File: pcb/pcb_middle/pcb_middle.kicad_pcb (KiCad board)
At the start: 2 copper layers, 37 x 37 mm, 25 parts, among them J1 MicroLab, J2 Pump 1, J3 Pump 2, Q1 NX7002BKR, Q2 NX7002BKR, Q3 NX7002BKR

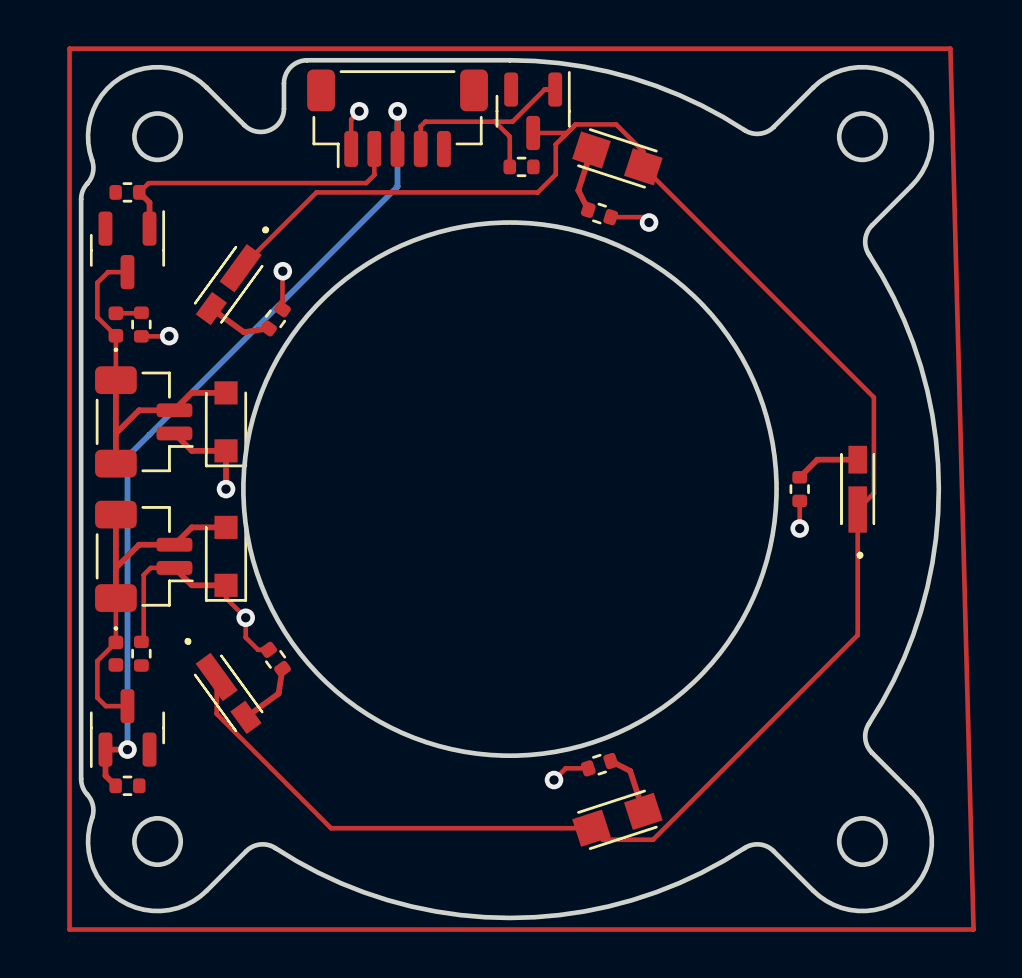
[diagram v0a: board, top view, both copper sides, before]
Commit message: fin
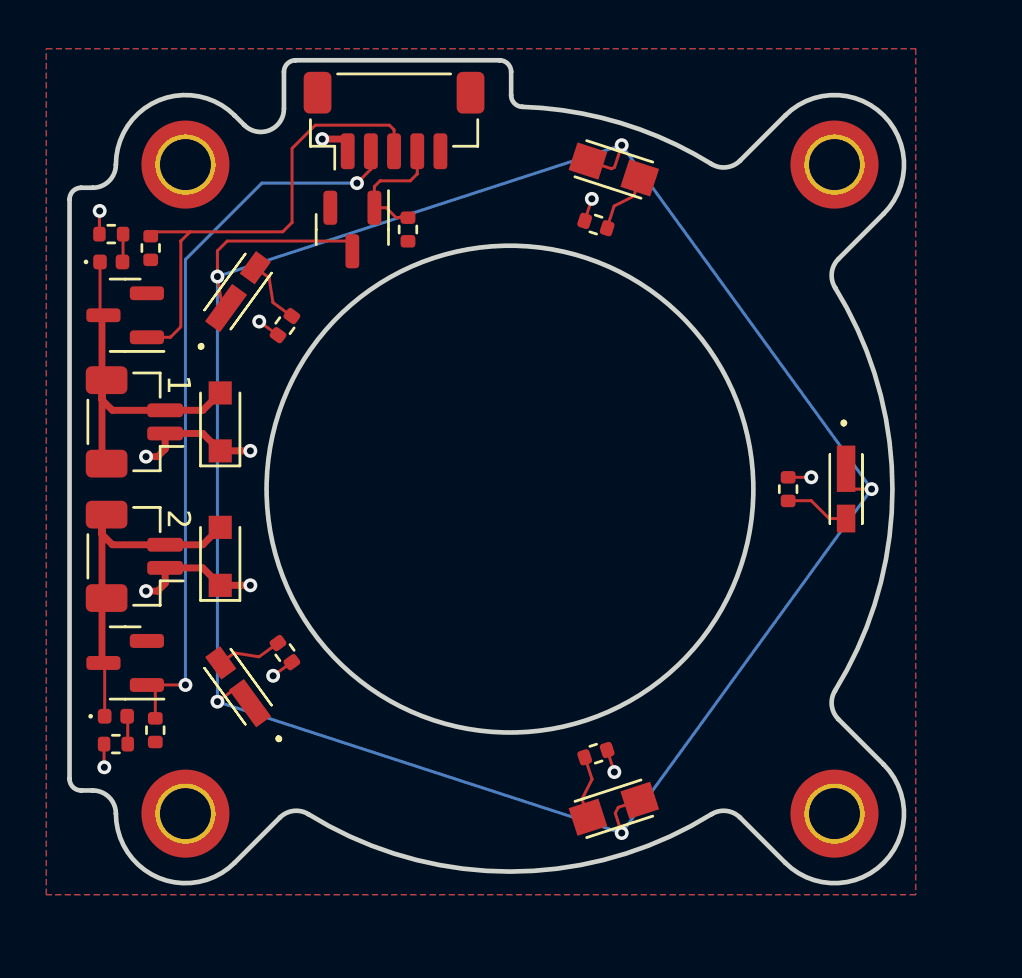
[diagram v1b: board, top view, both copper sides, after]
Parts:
- added H1: M2, MountingHole:MountingHole_2.2mm_M2_DIN965_Pad_TopOnly, F.Cu at (14.0, -14.0)
- added H2: M2, MountingHole:MountingHole_2.2mm_M2_DIN965_Pad_TopOnly, F.Cu at (14.0, 14.0)
- added H3: M2, MountingHole:MountingHole_2.2mm_M2_DIN965_Pad_TopOnly, F.Cu at (-14.0, 14.0)
- added H4: M2, MountingHole:MountingHole_2.2mm_M2_DIN965_Pad_TopOnly, F.Cu at (-14.0, -14.0)
- moved R7 23.2 mm to (-15.3, 10.4), turned to -90 degrees
- moved R2 23.2 mm to (-15.5, -10.4), turned to -90 degrees
- moved R9 18.1 mm to (-17.2, -11.0), turned to 0 degrees
- moved R10 18.1 mm to (-17.0, 11.0), turned to 0 degrees
- moved Q1 17.8 mm to (-16.6, -7.50), turned to 180 degrees
- moved Q3 17.8 mm to (-16.6, 7.50), turned to 180 degrees
- moved D2 17.3 mm to (-11.7, -8.52), turned to -126 degrees
- moved D4 17.3 mm to (-11.7, 8.52), turned to -54 degrees
- moved D8 16.9 mm to (-17.2, -9.80), turned to 0 degrees
- moved D9 16.9 mm to (-17.0, 9.80), turned to 0 degrees
- moved R3 14.4 mm to (-9.71, -7.05), turned to 54 degrees
- moved R4 14.4 mm to (-9.71, 7.05), turned to 126 degrees
- moved Q2 9.32 mm to (-6.80, -11.2)
- moved J2 5.81 mm to (-16.2, -2.90)
- moved J3 5.81 mm to (-16.2, 2.90)
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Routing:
- net (no net): track 153.0 -> 0.00 mm
- net Net-(D1-Pad1): track 83.7 -> 108.7 mm, vias 0 -> 5
- net /PUMP2_ON: track 13.3 -> 31.9 mm, vias 0 -> 2
- net /PUMP1_ON: track 36.7 -> 21.3 mm, vias 2 -> 0
- net /LED_ON: track 10.3 -> 5.59 mm
- net +5V: track 24.2 -> 19.6 mm, vias 8 -> 12
- net Net-(D8-Pad2): track 0.00 -> 1.21 mm
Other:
- board size 37 x 37 mm -> 36 x 35.5 mm
- board text added: "1"
- board text added: "2"
- board text added: "JLCJLCJLCJLC"
- board text added: "SAS SpaceLab 2023"
